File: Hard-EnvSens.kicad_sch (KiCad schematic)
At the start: 45 parts, among them P1 USB_C_Plug_USB2.0, SW1 SW_Push, SW3 SW_Push, U1 LD1117S33TR_SOT223, U2 ESP32-C6-WROOM-1, U3 CP2104, U4 VEML7700-TR, U5 DPS310, U6 SGP41-D-R4, U7 SHT40-AD1B-R2

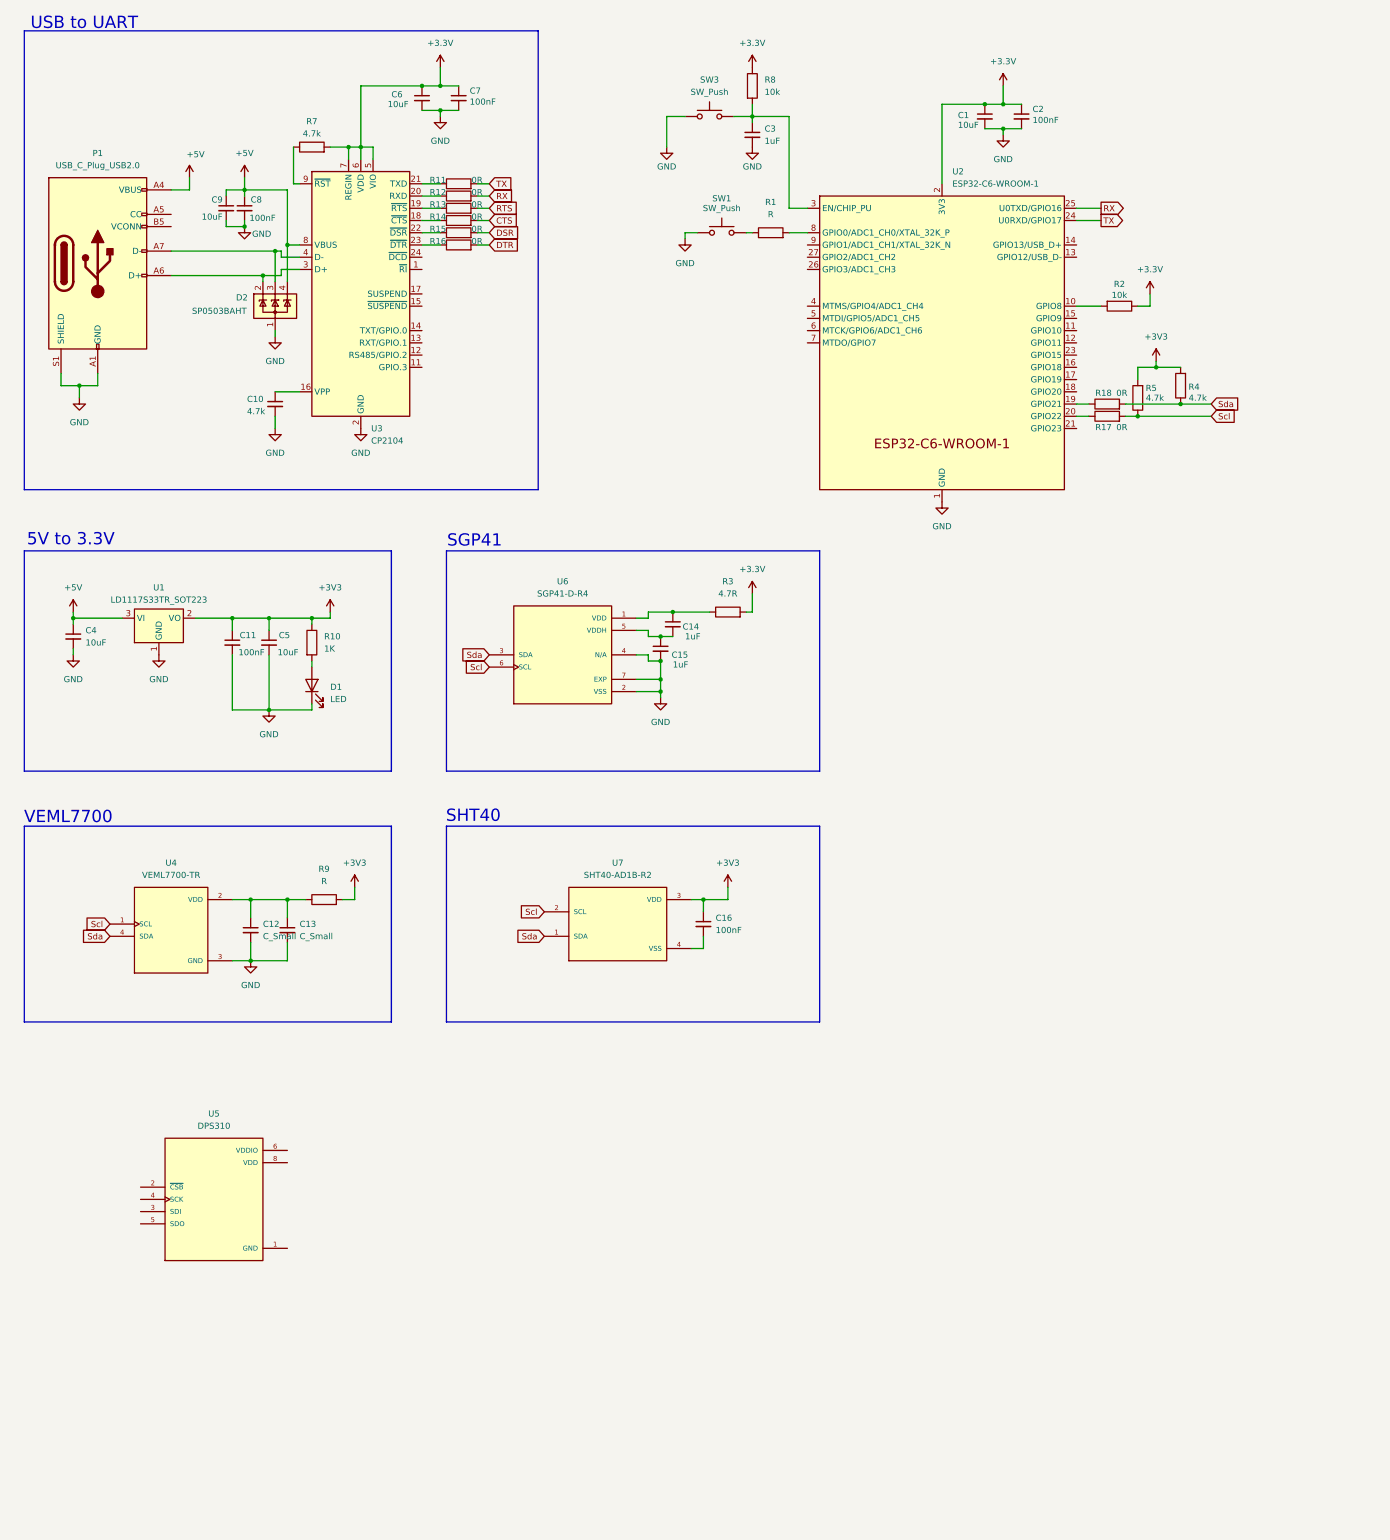
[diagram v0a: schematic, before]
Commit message: Dps368
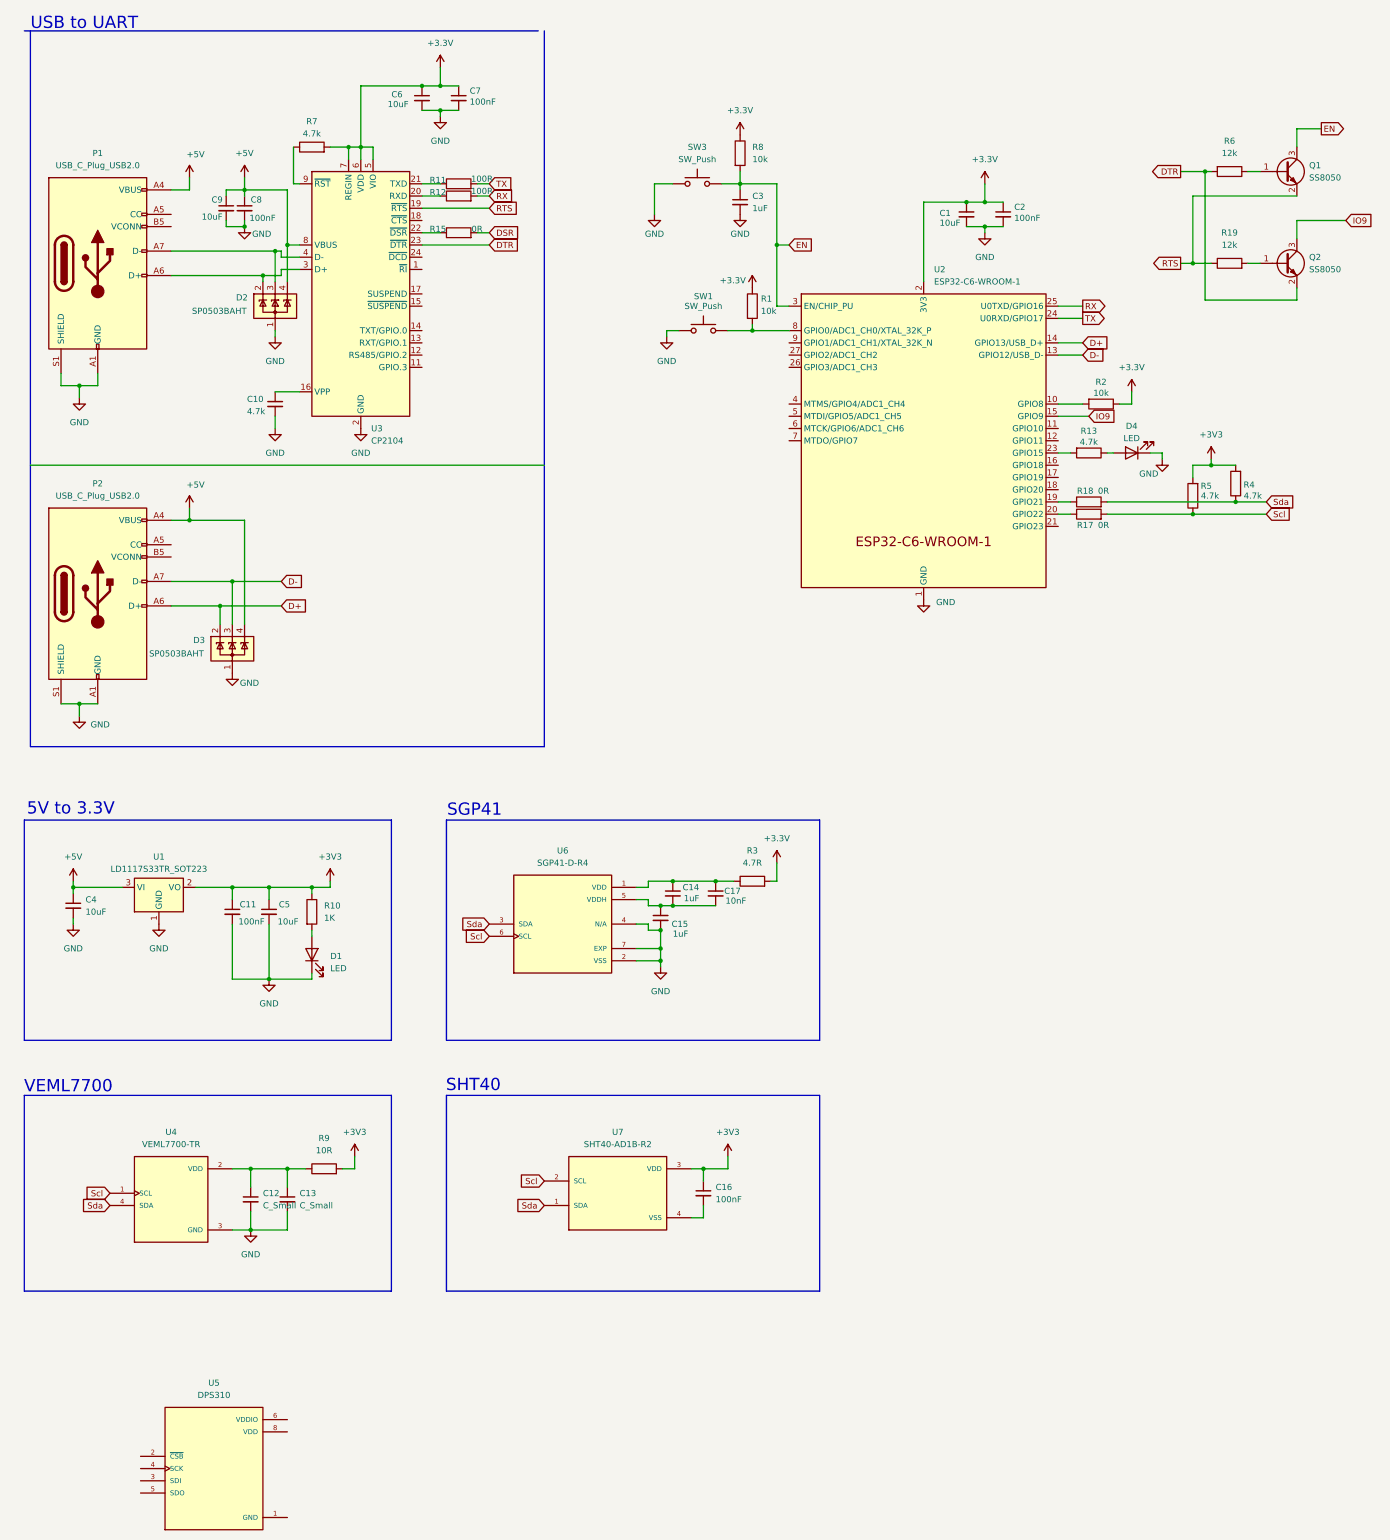
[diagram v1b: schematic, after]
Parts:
- removed R14, R16: 0R, symbol Device:R
- added C17: 10nF, symbol Device:C_Small
- added D3: SP0503BAHT, Package_TO_SOT_SMD:SOT-143, symbol Power_Protection:SP0503BAHT
- added D4: LED, symbol Device:LED
- added P2: USB_C_Plug_USB2.0, symbol Connector:USB_C_Plug_USB2.0
- added Q1, Q2: SS8050, Package_TO_SOT_SMD:SOT-23, symbol Transistor_BJT:SS8050
- added R19, R6: 12k, symbol Device:R
- R1: value R -> 10k
- R11, R12: value 0R -> 100R
- R13: value 0R -> 4.7k
- R9: value R -> 10R
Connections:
- net +3.3V: now also R1.1
- net +5V: now also D3.4 (K), P2.A4 (VBUS), P2.A9 (VBUS), P2.B4 (VBUS), P2.B9 (VBUS)
- net DTR: now also U3.23 (~{DTR}), Q2.2 (E), R6.2
- net GND: now also D3.1 (A), D4.1 (K), P2.A1 (GND), P2.A12 (GND), P2.B1 (GND), P2.B12 (GND), P2.S1 (SHIELD)
- net RTS: now also U3.19 (~{RTS}), Q1.2 (E), R19.1; no longer R13.2
- net EN: now reaches C3.1, R8.2, SW3.2, U2.3 (EN/CHIP_PU)
- net EN: now also Q1.3 (C)
- net at SW1.2: now also R1.2, U2.8 (GPIO0/ADC1_CH0/XTAL_32K_P); no longer R1.1
- net at C14.1, R3.1, U6.1 (VDD): now also C17.1
- net at R13.1: now also D4.2 (A); no longer U3.19 (~{RTS})
- net at C14.2, C15.1, U6.5 (VDDH): now also C17.2
- net D-: now reaches U2.13 (GPIO12/USB_D-)
- net D-: now also D3.3 (K), P2.A7 (D-)
- net D+: now reaches U2.14 (GPIO13/USB_D+)
- net D+: now also D3.2 (K), P2.A6 (D+)
- net IO9: now reaches U2.15 (GPIO9)
- net IO9: now also Q2.3 (C)
- net at U2.23 (GPIO15): now also R13.2
- new net: Q2.1 (B), R19.2
- new net: Q1.1 (B), R6.1
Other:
- moved on the sheet: C1, C11, C12, C13, C14, C15, C16, C2, C3, C4, C5, D1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
